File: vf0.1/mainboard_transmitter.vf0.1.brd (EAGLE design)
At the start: 58.4 x 38.1 mm, 15 parts, among them J2 U.FL, Y1 16MHz

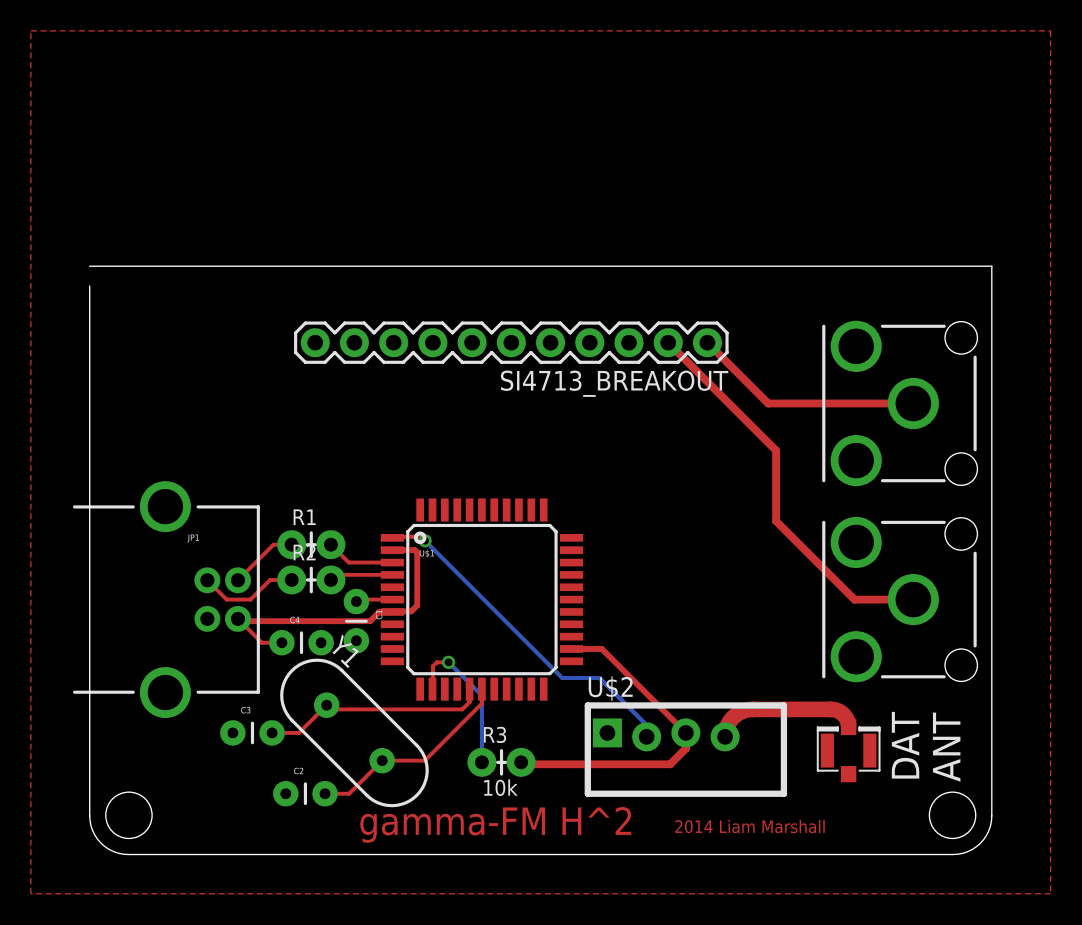
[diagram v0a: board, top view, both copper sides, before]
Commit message: Final revision of vf0.1
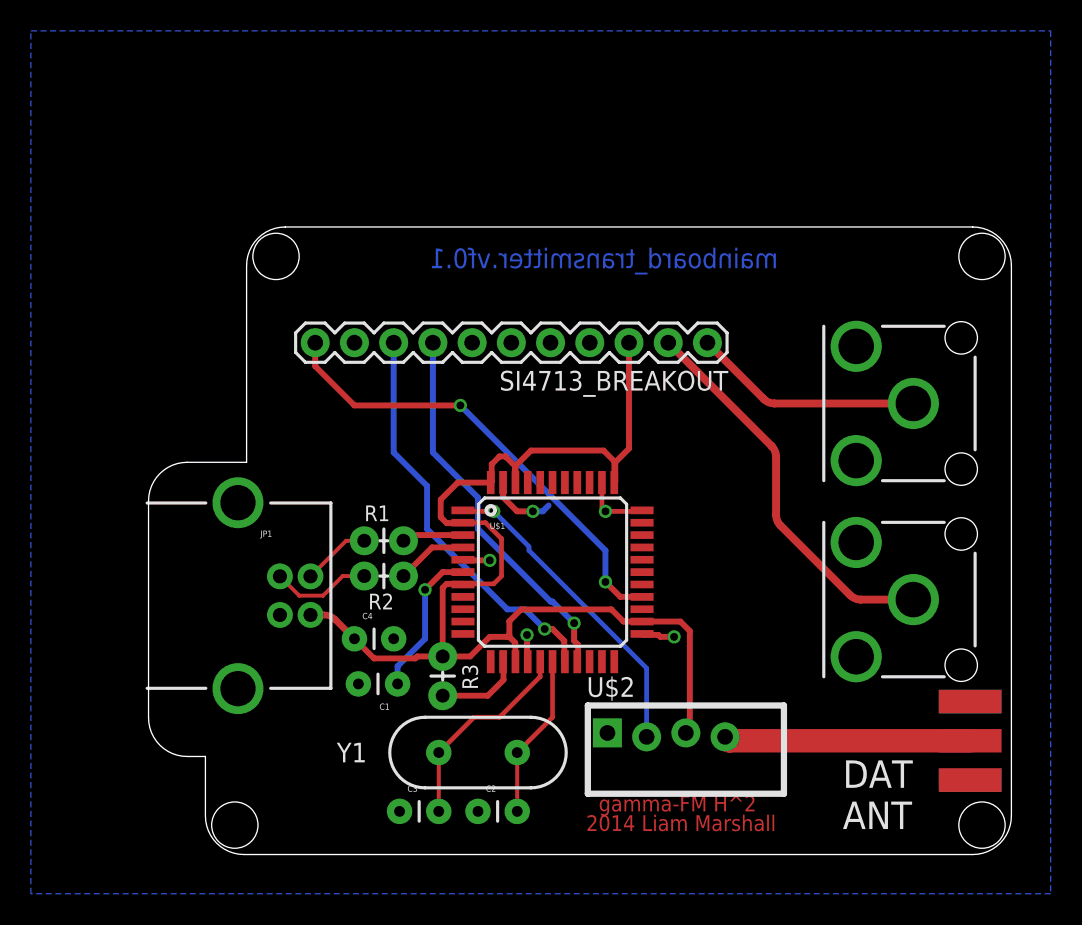
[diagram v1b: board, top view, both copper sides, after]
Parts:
- removed J2: U.FL, SparkFun-Connectors:U.FL
- added J$1: SMA_EDGE, SparkFun-Connectors:SMA-EDGE
- moved C2 12.5 mm to (25.1, 2.79)
- moved C3 11.9 mm to (20.1, 2.79)
- moved Y1 8.10 mm to (25.1, 6.60), turned to 0 degrees
- moved C1 5.96 mm to (19.9, 11.0), turned to 180 degrees
- moved R3 5.01 mm to (22.9, 10.3), turned to 90 degrees
- moved U$1 4.91 mm to (30.0, 18.3)
- moved R1 4.71 mm to (17.8, 20.3)
- moved C4 4.71 mm to (17.1, 14.0)
- moved R2 4.71 mm to (17.8, 18.0)
- moved JP1 4.71 mm to (12.3, 16.8)
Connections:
- removed net UVCC: C4.1, JP1.VBUS, U$1.2, U$1.7
- net GND: now also J$1.GND@0, J$1.GND@1, J$1.GND@2, J$1.GND@3; no longer J2.P$1, J2.P$2
- net N$9: now also J$1.SIG; no longer J2.P$3
- net VCC: now also C4.1, JP1.VBUS, U$1.2, U$1.7
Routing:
- net VCC: track 21.8 -> 80.4 mm
- net T_RST: track 0.00 -> 30.1 mm, vias 0 -> 2
- net SCL: track 0.00 -> 26.2 mm, vias 0 -> 1
- net SDA: track 0.00 -> 24.6 mm, vias 0 -> 1
- net UVCC: track 20.7 -> 0.00 mm
- net GND: track 0.00 -> 14.4 mm, vias 0 -> 5
- net N$5: track 2.38 -> 9.76 mm, vias 0 -> 1
- net N$9: track 9.21 -> 16.0 mm
- net N$8: track 9.98 -> 5.55 mm, vias 1 -> 0
- net N$6: track 13.5 -> 10.6 mm
- net RADIODAT: track 22.3 -> 20.7 mm
- net N$7: track 14.7 -> 13.4 mm
- net N$4: track 4.12 -> 4.62 mm
- added copper zone on layer 16, net GND
- removed copper zone on layer 1, net GND
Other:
- board size 58.4 x 38.1 mm -> 55.9 x 40.6 mm
- board text added: ">DRAWING_NAME"
